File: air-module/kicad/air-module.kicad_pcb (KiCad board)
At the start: 2 copper layers, 71.1 x 41.1 mm, 39 parts, among them J1 IDC12, J2 ARM_SWD_SMALL, P1 USB_OTG, U1 Alphasense_OPC-N2, U2 nRF52832, U3 Plantower_PM2.5_PMS_5003, U4 TPS2064, U5 BME280, U6 TPS79133

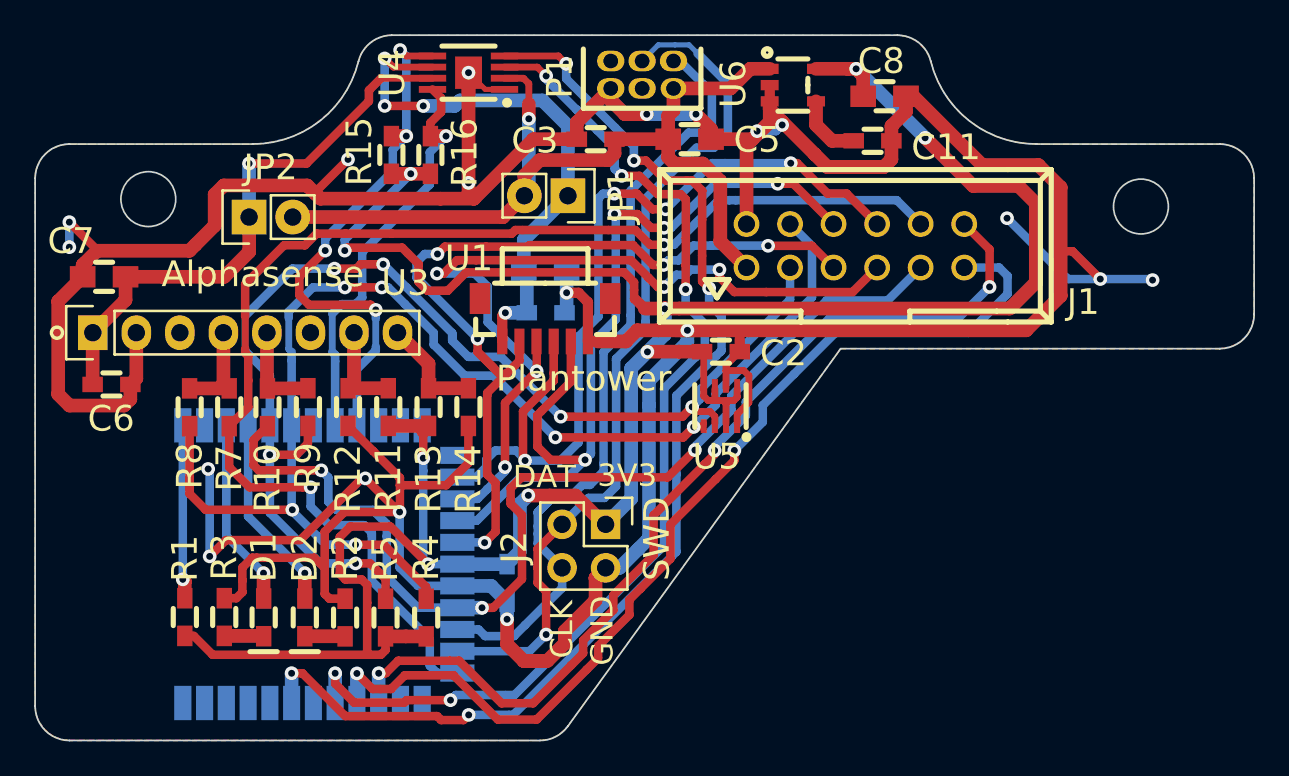
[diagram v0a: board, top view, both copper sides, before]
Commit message: Air Module PCB update
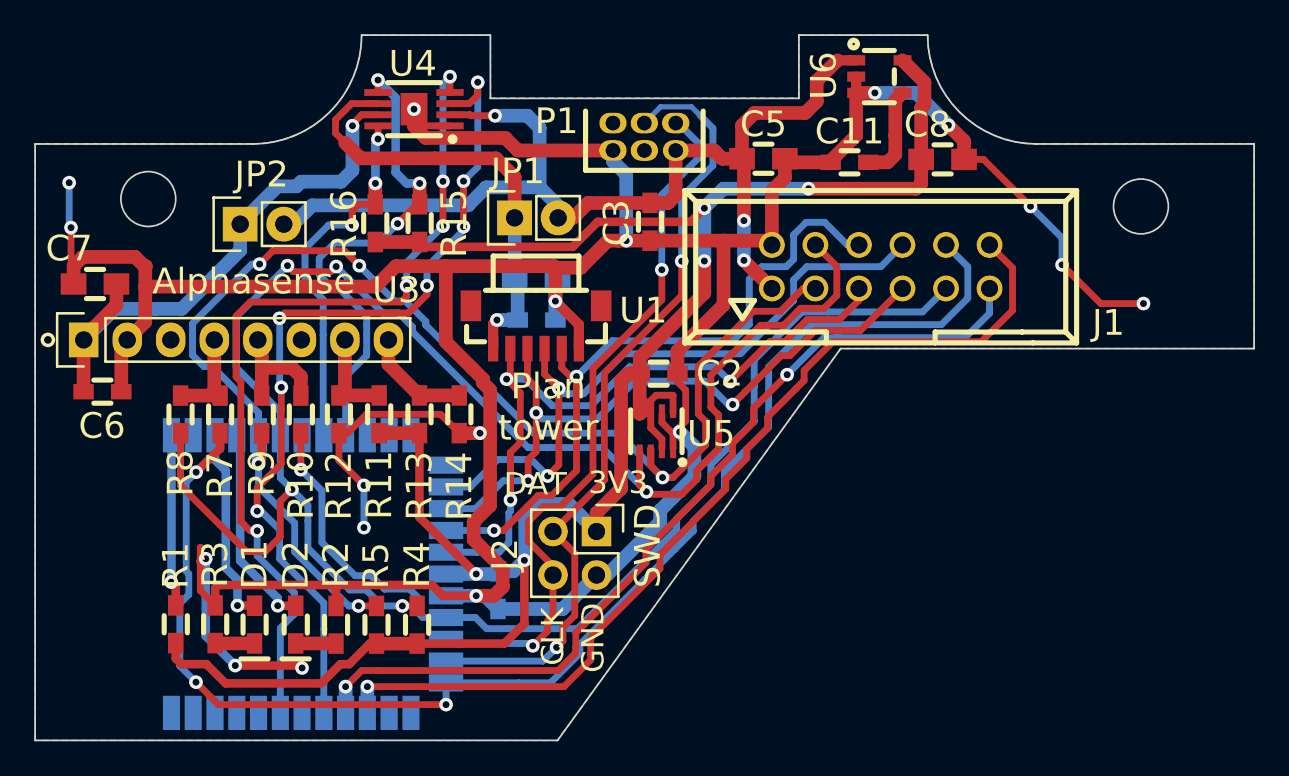
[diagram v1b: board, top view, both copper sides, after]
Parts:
- removed G***: LOGO, OPENHARDWARE:OSHWLOGO0.3IN
- moved C3 5.77 mm to (144.2, 87.8), turned to 270 degrees
- moved R16 5.12 mm to (128.2, 87.9)
- moved U6 5.07 mm to (156.2, 79.4)
- moved C8 5.00 mm to (161.3, 84.2)
- moved C5 4.46 mm to (150.8, 84.1)
- moved R15 4.31 mm to (130.8, 87.9)
- moved U5 4.02 mm to (143.3, 98.8)
- moved C2 3.86 mm to (144.7, 96.7)
- moved U4 3.83 mm to (130.4, 81.3)
- moved P1 3.62 mm to (143.9, 82.9)
- moved JP1 3.37 mm to (136.3, 87.6), turned to 0 degrees
- moved R9 2.72 mm to (121.6, 99.1)
- moved R10 1.99 mm to (123.8, 99.1)
- moved J1 1.92 mm to (156.4, 90.4)
- moved C11 1.84 mm to (155.9, 84.4), turned to 180 degrees
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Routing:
- net GND: track 282.3 -> 233.0 mm, vias 19 -> 18
- net +3V3: track 155.9 -> 124.2 mm, vias 9 -> 5
- net EN_ALPHA: track 67.8 -> 50.4 mm
- net TWI-SCL: track 77.6 -> 94.0 mm, vias 6 -> 5
- net SPI-MOSI: track 52.6 -> 39.5 mm, vias 4 -> 2
- net EN_PLANT: track 63.2 -> 50.8 mm, vias 5 -> 7
- net SPI-MISO: track 49.7 -> 39.4 mm, vias 5 -> 3
- net SPI-CS: track 49.2 -> 39.9 mm, vias 4 -> 2
- net TWI-SDA: track 69.5 -> 78.5 mm, vias 6 -> 5
- net +5V: track 52.7 -> 60.6 mm, vias 1 -> 3
- net SPI-SCLK: track 51.2 -> 43.4 mm, vias 5 -> 3
- net MCU-CTS: track 58.5 -> 51.9 mm
- net VCC_ALPHA: track 32.4 -> 26.5 mm, vias 4 -> 1
- net TCK: track 46.7 -> 42.3 mm, vias 0 -> 2
- net MCU-RX: track 75.4 -> 79.1 mm, vias 2 -> 3
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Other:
- outline, holes or cut-outs redrawn
- board text added: "Plan tower"
- board text removed: "Plantower"
